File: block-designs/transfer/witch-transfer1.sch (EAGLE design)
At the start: 18 parts, among them IC1 74LS73N, IC2 74S08N

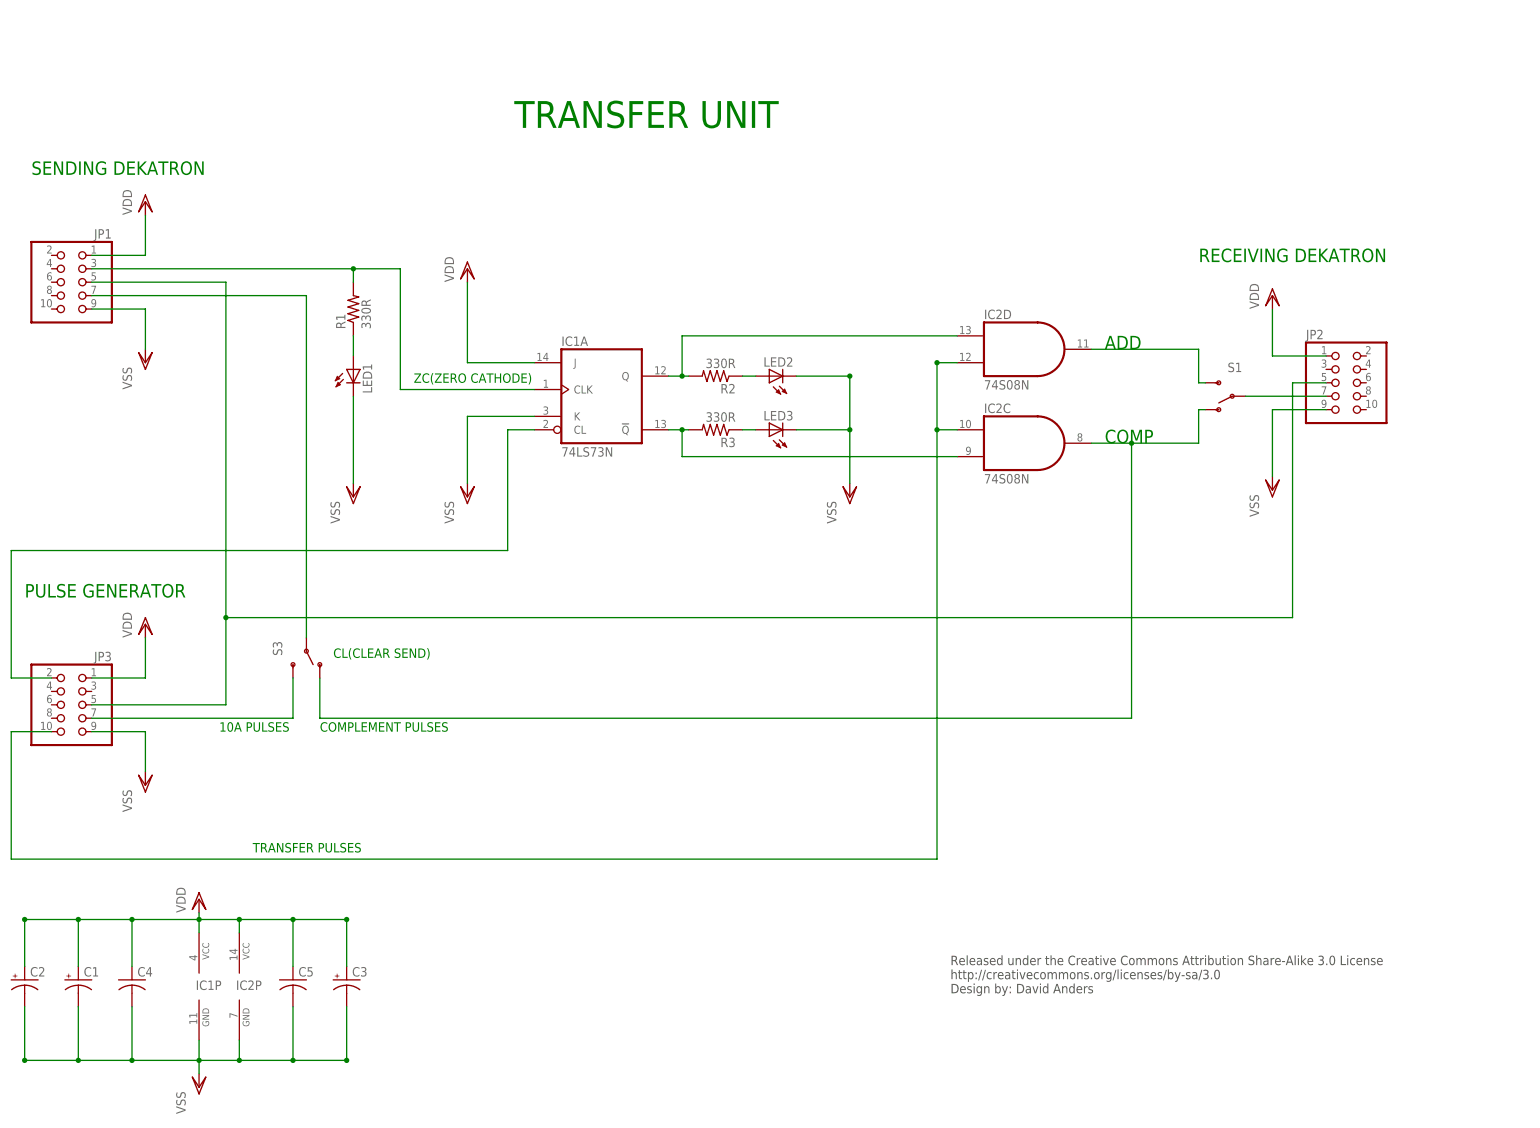
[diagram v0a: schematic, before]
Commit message: updated files with new images
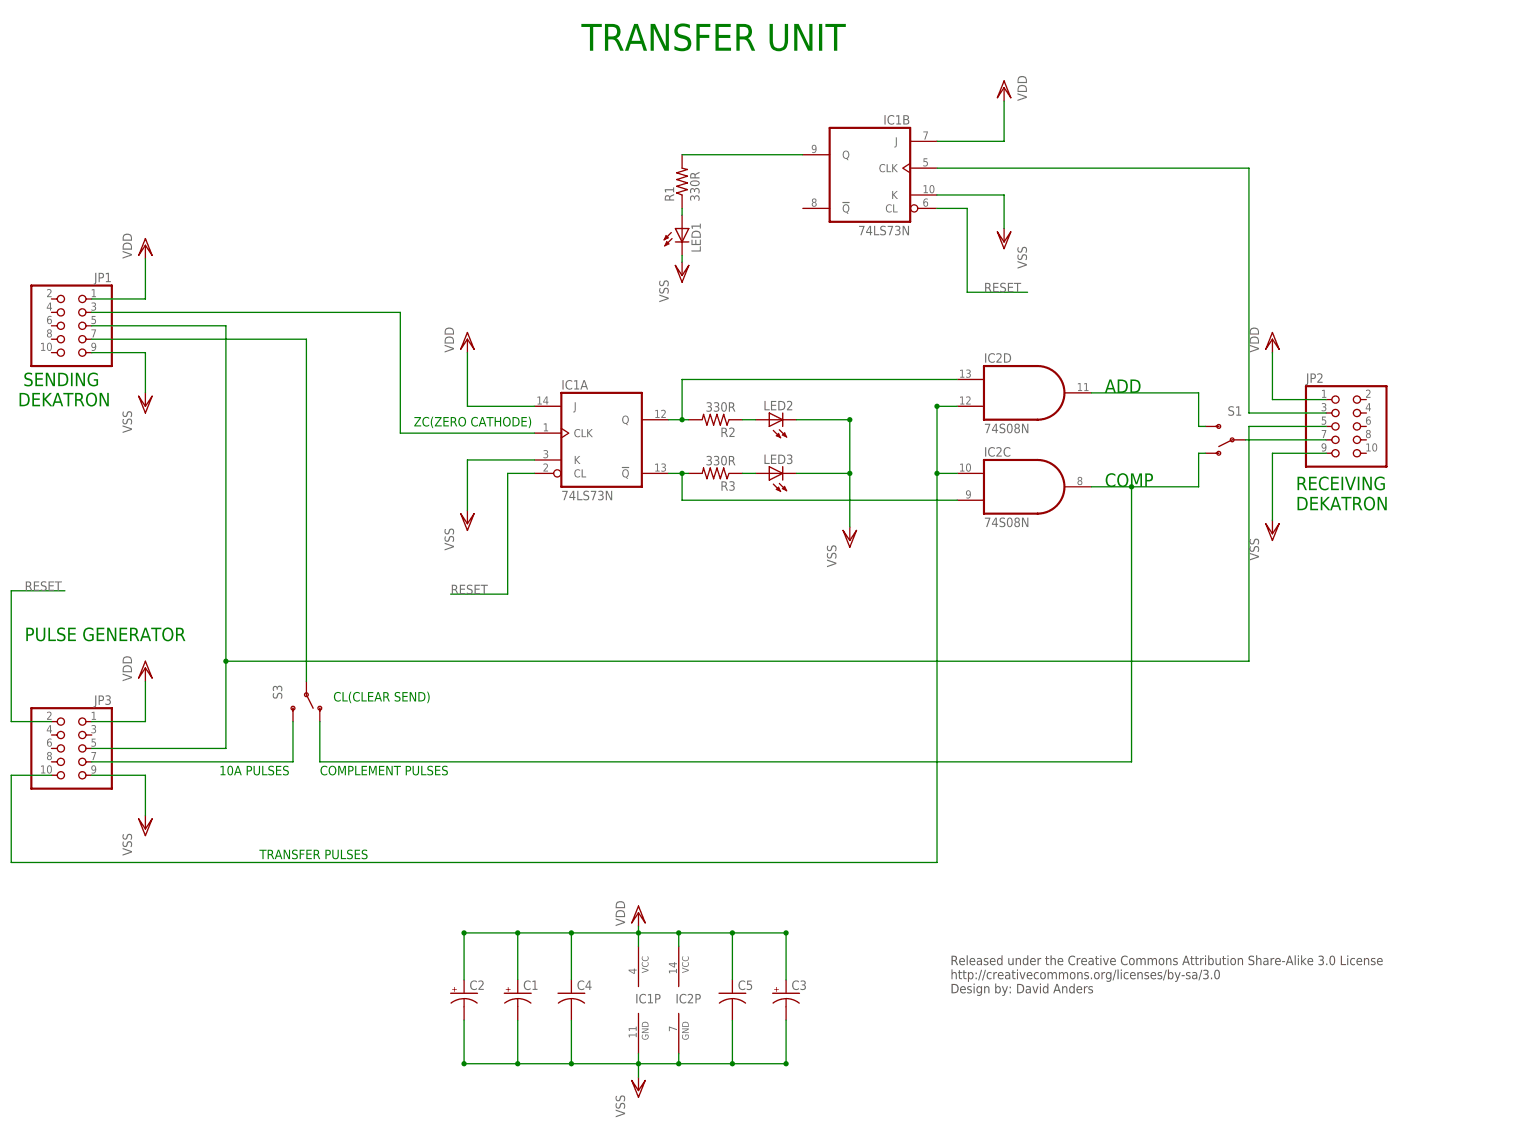
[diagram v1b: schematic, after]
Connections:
- removed net N$10: IC1A.CL, JP3.2
- new net N$11: IC1B.CLK, JP2.3
- new net N$12: IC1B.Q, R1.2
- new net RESET: IC1A.CL, IC1B.CL, JP3.2
- net VDD: now also IC1B.J
- net VSS: now also IC1B.K
- net ZC_TX: no longer R1.2
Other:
- moved on the sheet: C1, C2, C3, C4, C5, IC1A, IC1P, IC2C, IC2D, IC2P, JP1, JP2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
